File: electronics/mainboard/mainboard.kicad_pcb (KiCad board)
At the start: 2 copper layers, 3 parts, among them J1 Conn_01x09, J2 Conn_01x09

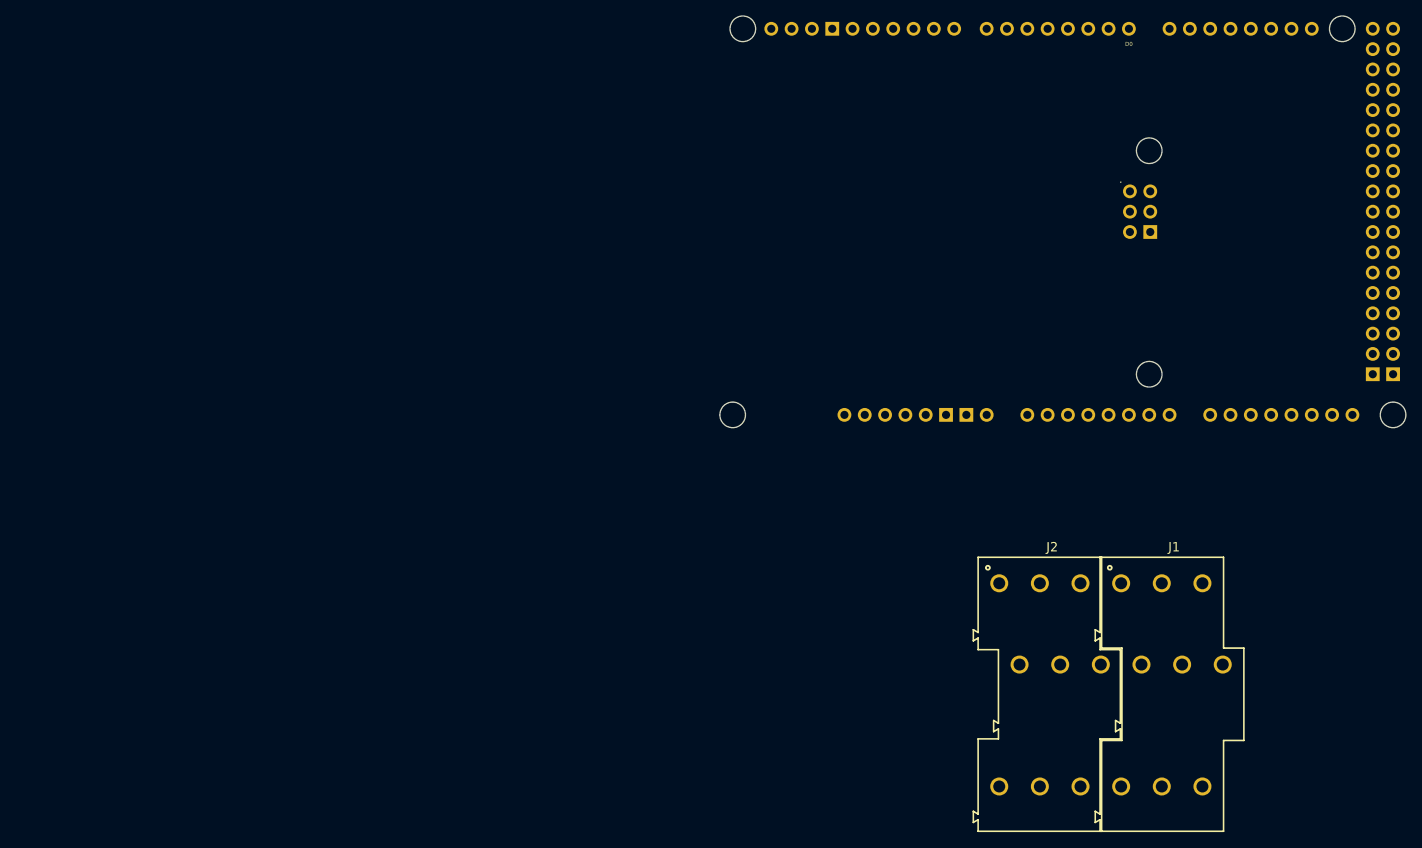
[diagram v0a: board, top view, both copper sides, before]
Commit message: place parts
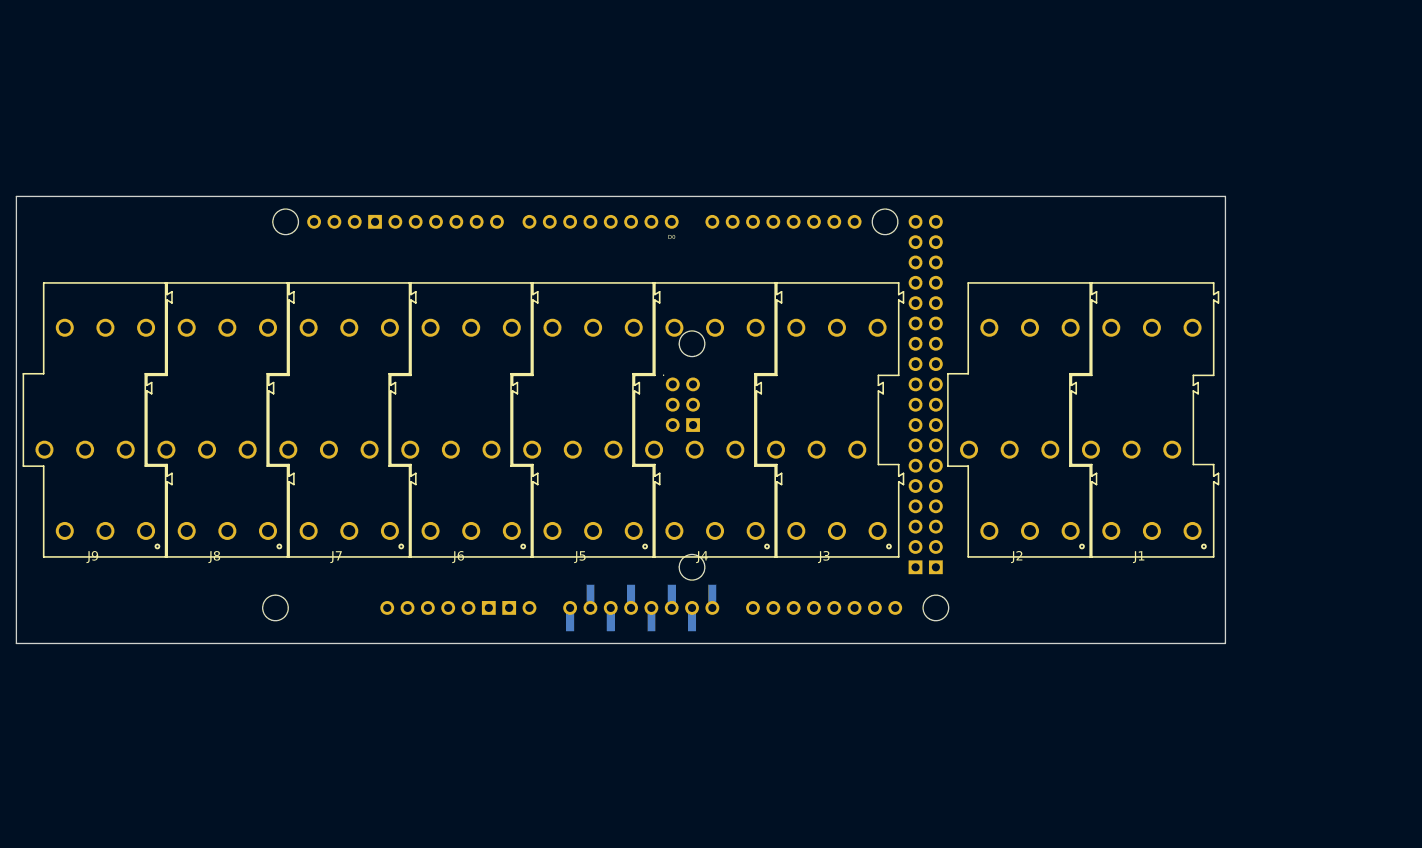
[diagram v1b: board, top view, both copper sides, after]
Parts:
- added J3: Conn_01x09, Wuerth:691247510009, F.Cu at (178.8, 91.3)
- added J4: Conn_01x09, Wuerth:691247510009, F.Cu at (163.5, 91.3)
- added J5: Conn_01x09, Wuerth:691247510009, F.Cu at (148.3, 91.3)
- added J6: Conn_01x09, Wuerth:691247510009, F.Cu at (133.1, 91.3)
- added J7: Conn_01x09, Wuerth:691247510009, F.Cu at (117.8, 91.3)
- added J8: Conn_01x09, Wuerth:691247510009, F.Cu at (102.6, 91.3)
- added J9: Conn_01x09, Wuerth:691247510009, F.Cu at (87.3, 91.3)
- added J99: Conn_01x08, Connector_PinHeader_2.54mm:PinHeader_1x08_P2.54mm_Vertical_SMD_Pin1Right, B.Cu at (156.8, 111.1)
- moved XA1 62.0 mm to (97.2, 113.7)
- moved J1 27.6 mm to (218.1, 91.3), turned to 180 degrees
- moved J2 27.6 mm to (202.9, 91.3), turned to 180 degrees
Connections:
- XA1 pad A0: unconnected-(XA1-PadA0) -> Net-(XA1-PadA0)
- XA1 pad A1: unconnected-(XA1-PadA1) -> Net-(XA1-PadA1)
- XA1 pad A2: unconnected-(XA1-PadA2) -> Net-(XA1-PadA2)
- XA1 pad A3: unconnected-(XA1-PadA3) -> Net-(XA1-PadA3)
- XA1 pad A4: unconnected-(XA1-PadA4) -> Net-(XA1-PadA4)
- XA1 pad A5: unconnected-(XA1-PadA5) -> Net-(XA1-PadA5)
- XA1 pad A6: unconnected-(XA1-PadA6) -> Net-(XA1-PadA6)
- XA1 pad A7: unconnected-(XA1-PadA7) -> Net-(XA1-PadA7)
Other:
- board outline added: 151.1 x 55.9 mm
